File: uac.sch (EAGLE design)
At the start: 206 parts, among them Q6 2N7002CK4SST, Q7 2N7002CK4SST, U2 ADXL345, Y1 RESONATORSMD

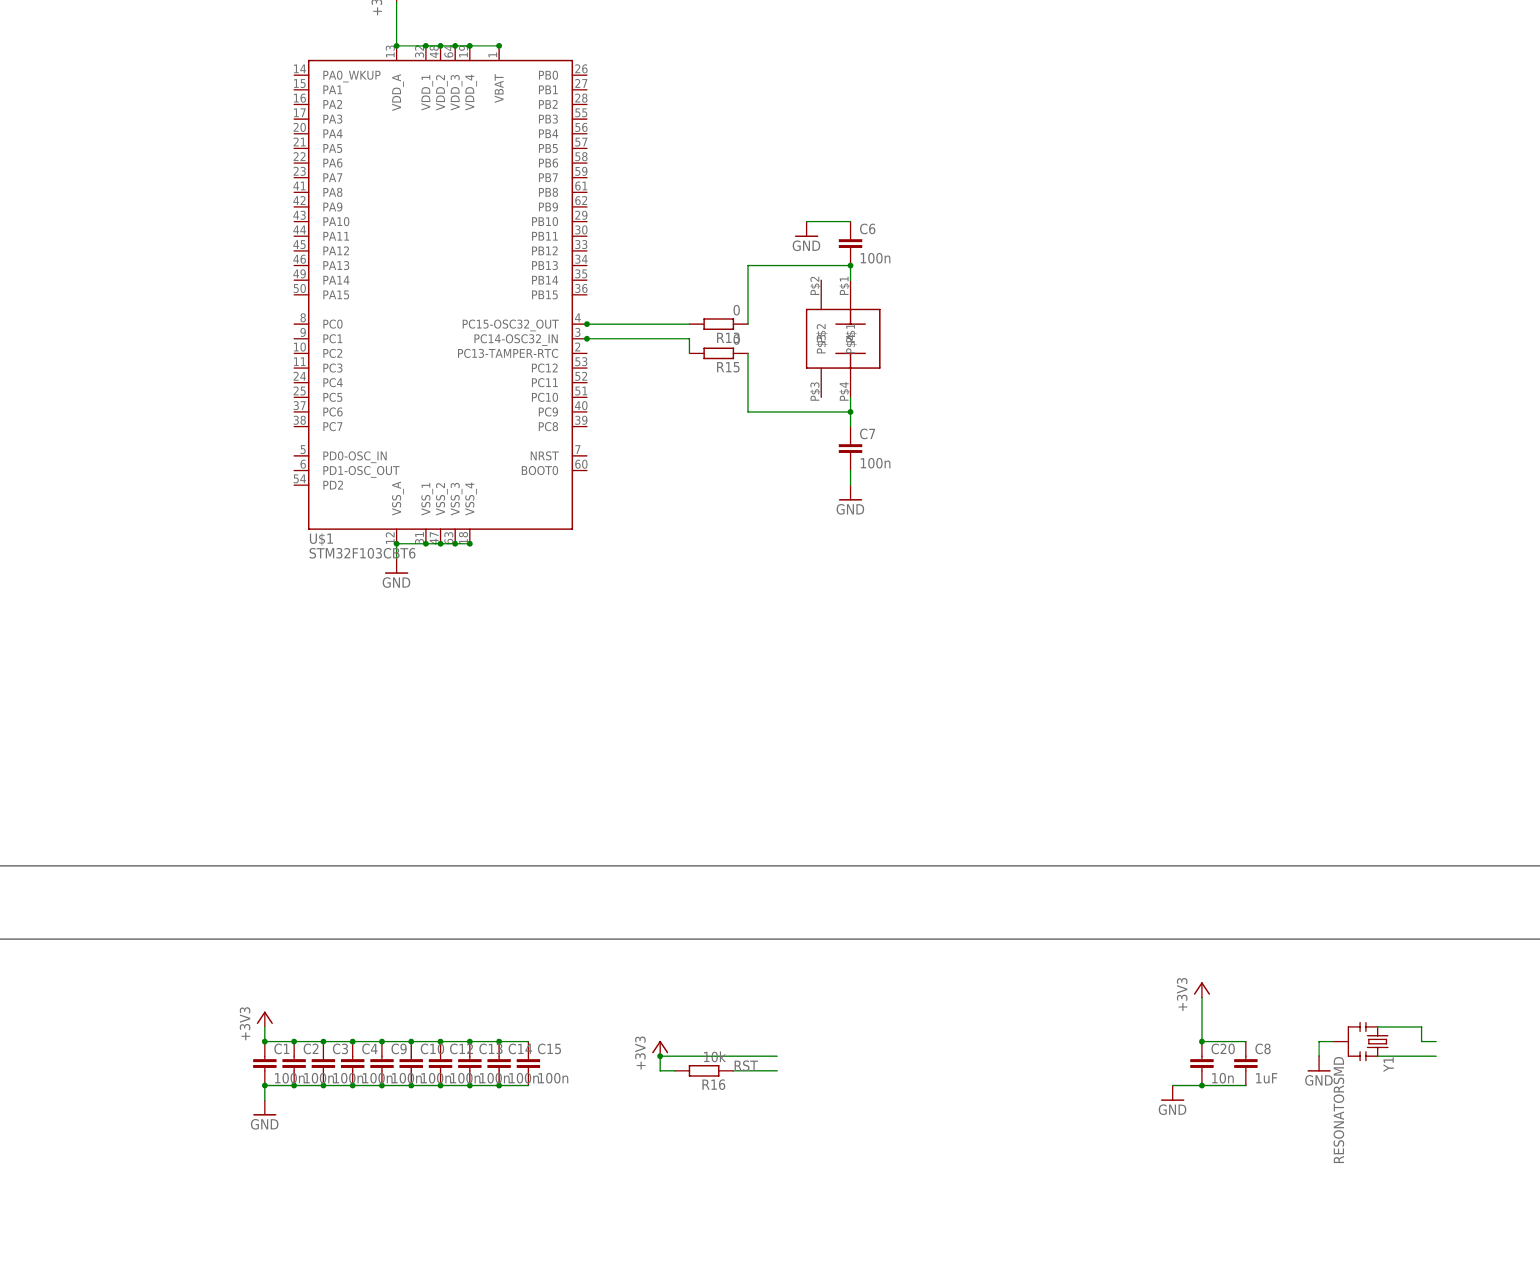
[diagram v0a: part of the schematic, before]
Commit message: connecting
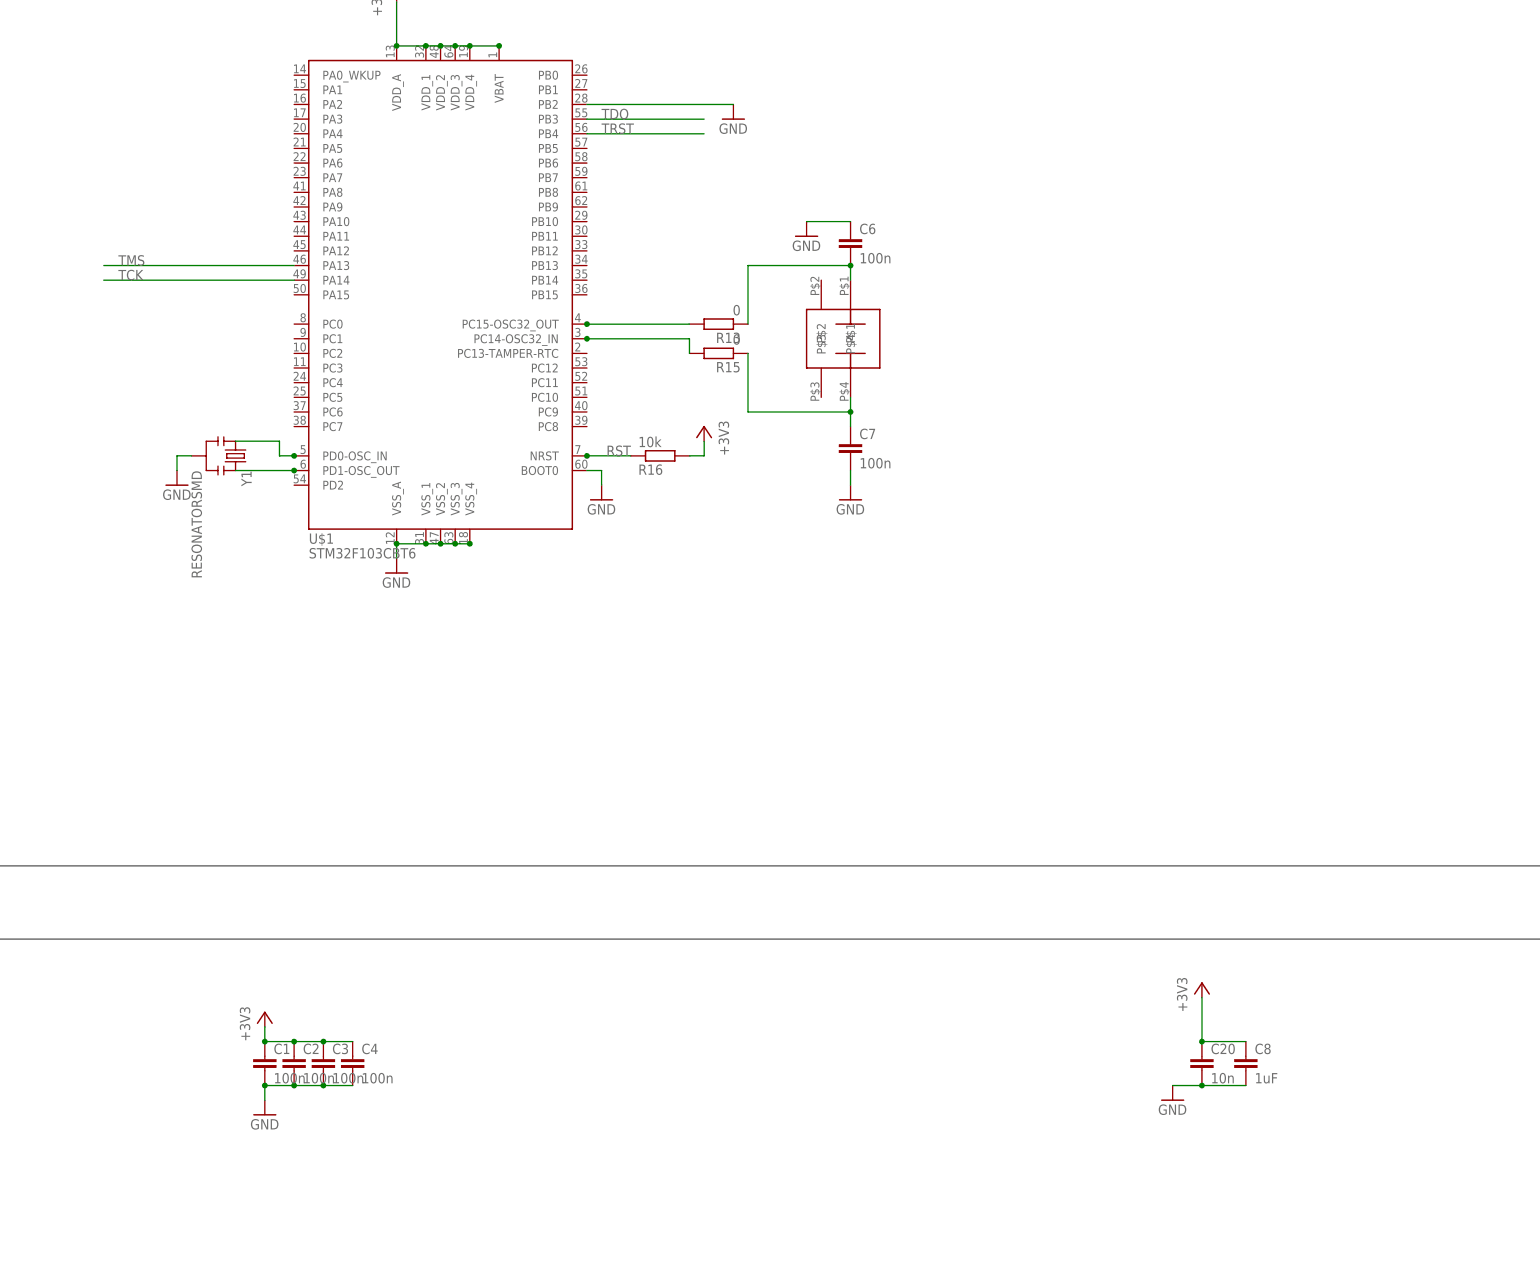
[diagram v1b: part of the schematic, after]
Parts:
- removed C10, C12, C13, C14, C15, C9: 100n, Custom components:C-EUC0603
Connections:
- net +3V3: no longer C10.1, C12.1, C13.1, C14.1, C15.1, C9.1
- net GND: now also U$1.BOOT0, U$1.PB2; no longer C10.2, C12.2, C13.2, C14.2, C15.2, C9.2
- net N$1: now also U$1.PD1-OSC_OUT
- net N$2: now also U$1.PD0-OSC_IN
- net RST: now also U$1.NRST
- net TCK: now also U$1.PA14
- net TDO: now also U$1.PB3
- net TMS: now also U$1.PA13
- net TRST: now also U$1.PB4
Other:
- moved on the sheet: R16, Y1
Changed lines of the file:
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@@
 <part name="+3V7" library="supply1" deviceset="+3V3" device=""/>
 <part name="R16" library="Custom components" deviceset="R-EU_" device="R0603" value="10k"/>
-<part name="C9" library="Custom components" deviceset="C-EU" device="C0603" value="100n"/>
-<part name="C10" library="Custom components" deviceset="C-EU" device="C0603" value="100n"/>
-<part name="C12" library="Custom components" deviceset="C-EU" device="C0603" value="100n"/>
-<part name="C13" library="Custom components" deviceset="C-EU" device="C0603" value="100n"/>
-<part name="C14" library="Custom components" deviceset="C-EU" device="C0603" value="100n"/>
-<part name="C15" library="Custom components" deviceset="C-EU" device="C0603" value="100n"/>
 <part name="GND4" library="supply1" deviceset="GND" device=""/>
 <part name="C18" library="Custom components" deviceset="C-EU" device="C0603" value="100n"/>
@@
 <part name="JP1" library="SparkFun2012" deviceset="JUMPER-2" device="SMD-NO"/>
 <part name="U$1" library="stm32" deviceset="STM32F103CBT6" device=""/>
+<part name="GND3" library="Custom components" deviceset="GND" device=""/>
+<part name="GND5" library="Custom components" deviceset="GND" device=""/>
 </parts>
 <sheets>
@@
 <instance part="C4" gate="G$1" x="147.32" y="215.9"/>
 <instance part="+3V2" gate="G$1" x="132.08" y="223.52"/>
-<instance part="Y1" gate="G$1" x="325.12" y="218.44" rot="R270"/>
-<instance part="GND2" gate="1" x="314.96" y="213.36"/>
+<instance part="Y1" gate="G$1" x="127" y="320.04" rot="R270"/>
+<instance part="GND2" gate="1" x="116.84" y="314.96"/>
 <instance part="MASTER_PROG" gate="A" x="35.56" y="203.2"/>
 <instance part="GND19" gate="1" x="12.7" y="208.28"/>
@@
 <instance part="+3V5" gate="G$1" x="154.94" y="401.32"/>
 <instance part="GND9" gate="1" x="154.94" y="299.72"/>
-<instance part="+3V7" gate="G$1" x="200.66" y="218.44"/>
-<instance part="R16" gate="G$1" x="208.28" y="213.36" rot="R180"/>
-<instance part="C9" gate="G$1" x="152.4" y="215.9"/>
-<instance part="C10" gate="G$1" x="157.48" y="215.9"/>
-<instance part="C12" gate="G$1" x="162.56" y="215.9"/>
-<instance part="C13" gate="G$1" x="167.64" y="215.9"/>
-<instance part="C14" gate="G$1" x="172.72" y="215.9"/>
-<instance part="C15" gate="G$1" x="177.8" y="215.9"/>
+<instance part="+3V7" gate="G$1" x="208.28" y="325.12" rot="MR0"/>
+<instance part="R16" gate="G$1" x="200.66" y="320.04" rot="MR180"/>
 <instance part="GND4" gate="1" x="38.1" y="20.32"/>
 <instance part="C18" gate="G$1" x="48.26" y="38.1"/>
@@
 <instance part="JP1" gate="A" x="419.1" y="134.62"/>
 <instance part="U$1" gate="G$1" x="149.86" y="363.22"/>
+<instance part="GND3" gate="1" x="190.5" y="312.42"/>
+<instance part="GND5" gate="1" x="213.36" y="378.46"/>
 </instances>
 <busses>
@@
 <pinref part="Y1" gate="G$1" pin="2"/>
 <pinref part="GND2" gate="1" pin="GND"/>
-<wire x1="317.5" y1="218.44" x2="314.96" y2="218.44" width="0.1524" layer="91"/>
-<wire x1="314.96" y1="218.44" x2="314.96" y2="215.9" width="0.1524" layer="91"/>
+<wire x1="119.38" y1="320.04" x2="116.84" y2="320.04" width="0.1524" layer="91"/>
+<wire x1="116.84" y1="320.04" x2="116.84" y2="317.5" width="0.1524" layer="91"/>
 </segment>
 <segment>
@@
 <junction x="137.16" y="210.82"/>
 <junction x="142.24" y="210.82"/>
-<junction x="147.32" y="210.82"/>
 <pinref part="GND1" gate="1" pin="GND"/>
 <wire x1="132.08" y1="208.28" x2="132.08" y2="210.82" width="0.1524" layer="91"/>
 <junction x="132.08" y="210.82"/>
-<pinref part="C15" gate="G$1" pin="2"/>
-<pinref part="C14" gate="G$1" pin="2"/>
-<wire x1="177.8" y1="210.82" x2="172.72" y2="210.82" width="0.1524" layer="91"/>
-<pinref part="C13" gate="G$1" pin="2"/>
-<wire x1="172.72" y1="210.82" x2="167.64" y2="210.82" width="0.1524" layer="91"/>
-<pinref part="C12" gate="G$1" pin="2"/>
-<wire x1="167.64" y1="210.82" x2="162.56" y2="210.82" width="0.1524" layer="91"/>
-<pinref part="C10" gate="G$1" pin="2"/>
-<wire x1="162.56" y1="210.82" x2="157.48" y2="210.82" width="0.1524" layer="91"/>
-<pinref part="C9" gate="G$1" pin="2"/>
-<wire x1="157.48" y1="210.82" x2="152.4" y2="210.82" width="0.1524" layer="91"/>
-<wire x1="152.4" y1="210.82" x2="147.32" y2="210.82" width="0.1524" layer="91"/>
-<junction x="172.72" y="210.82"/>
-<junction x="167.64" y="210.82"/>
-<junction x="162.56" y="210.82"/>
-<junction x="157.48" y="210.82"/>
-<junction x="152.4" y="210.82"/>
 </segment>
 <segment>
@@
 <junction x="167.64" y="304.8"/>
 </segment>
+<segment>
+<pinref part="U$1" gate="G$1" pin="BOOT0"/>
+<pinref part="GND3" gate="1" pin="GND"/>
+<wire x1="187.96" y1="317.5" x2="190.5" y2="317.5" width="0.1524" layer="91"/>
+<wire x1="190.5" y1="317.5" x2="190.5" y2="314.96" width="0.1524" layer="91"/>
+</segment>
+<segment>
+<pinref part="U$1" gate="G$1" pin="PB2"/>
+<pinref part="GND5" gate="1" pin="GND"/>
+<wire x1="187.96" y1="381" x2="213.36" y2="381" width="0.1524" layer="91"/>
+</segment>
 </net>
 <net name="+3V3" class="0">
@@
 <segment>
 <pinref part="+3V7" gate="G$1" pin="+3V3"/>
-<wire x1="220.98" y1="215.9" x2="200.66" y2="215.9" width="0.1524" layer="91"/>
 <pinref part="R16" gate="G$1" pin="2"/>
-<wire x1="203.2" y1="213.36" x2="200.66" y2="213.36" width="0.1524" layer="91"/>
-<wire x1="200.66" y1="213.36" x2="200.66" y2="215.9" width="0.1524" layer="91"/>
-<junction x="200.66" y="215.9"/>
+<wire x1="205.74" y1="320.04" x2="208.28" y2="320.04" width="0.1524" layer="91"/>
+<wire x1="208.28" y1="320.04" x2="208.28" y2="322.58" width="0.1524" layer="91"/>
 </segment>
 <segment>
@@
 <wire x1="132.08" y1="220.98" x2="132.08" y2="218.44" width="0.1524" layer="91"/>
 <junction x="132.08" y="218.44"/>
-<pinref part="C9" gate="G$1" pin="1"/>
-<wire x1="147.32" y1="218.44" x2="152.4" y2="218.44" width="0.1524" layer="91"/>
-<pinref part="C10" gate="G$1" pin="1"/>
-<wire x1="152.4" y1="218.44" x2="157.48" y2="218.44" width="0.1524" layer="91"/>
-<pinref part="C12" gate="G$1" pin="1"/>
-<wire x1="157.48" y1="218.44" x2="162.56" y2="218.44" width="0.1524" layer="91"/>
-<pinref part="C13" gate="G$1" pin="1"/>
-<wire x1="162.56" y1="218.44" x2="167.64" y2="218.44" width="0.1524" layer="91"/>
-<pinref part="C14" gate="G$1" pin="1"/>
-<wire x1="167.64" y1="218.44" x2="172.72" y2="218.44" width="0.1524" layer="91"/>
-<pinref part="C15" gate="G$1" pin="1"/>
-<wire x1="172.72" y1="218.44" x2="177.8" y2="218.44" width="0.1524" layer="91"/>
-<junction x="147.32" y="218.44"/>
-<junction x="152.4" y="218.44"/>
-<junction x="157.48" y="218.44"/>
-<junction x="162.56" y="218.44"/>
-<junction x="167.64" y="218.44"/>
-<junction x="172.72" y="218.44"/>
 </segment>
 <segment>
@@
 <segment>
 <pinref part="Y1" gate="G$1" pin="3"/>
-<wire x1="335.28" y1="215.9" x2="325.12" y2="215.9" width="0.1524" layer="91"/>
+<wire x1="137.16" y1="317.5" x2="127" y2="317.5" width="0.1524" layer="91"/>
+<pinref part="U$1" gate="G$1" pin="PD1-OSC_OUT"/>
+<junction x="137.16" y="317.5"/>
 </segment>
 </net>
 <net name="N$2" class="0">
 <segment>
-<wire x1="335.28" y1="218.44" x2="332.74" y2="218.44" width="0.1524" layer="91"/>
-<wire x1="332.74" y1="218.44" x2="332.74" y2="220.98" width="0.1524" layer="91"/>
+<wire x1="137.16" y1="320.04" x2="134.62" y2="320.04" width="0.1524" layer="91"/>
+<wire x1="134.62" y1="320.04" x2="134.62" y2="322.58" width="0.1524" layer="91"/>
 <pinref part="Y1" gate="G$1" pin="1"/>
-<wire x1="332.74" y1="220.98" x2="325.12" y2="220.98" width="0.1524" layer="91"/>
+<wire x1="134.62" y1="322.58" x2="127" y2="322.58" width="0.1524" layer="91"/>
+<pinref part="U$1" gate="G$1" pin="PD0-OSC_IN"/>
+<junction x="137.16" y="320.04"/>
 </segment>
 </net>
@@
 <label x="22.86" y="142.24" size="1.778" layer="95"/>
 </segment>
+<segment>
+<pinref part="U$1" gate="G$1" pin="PA13"/>
+<wire x1="137.16" y1="353.06" x2="104.14" y2="353.06" width="0.1524" layer="91"/>
+<label x="106.68" y="353.06" size="1.778" layer="95"/>
+</segment>
 </net>
 <net name="TCK" class="0">
@@
 <label x="22.86" y="139.7" size="1.778" layer="95"/>
 </segment>
+<segment>
+<pinref part="U$1" gate="G$1" pin="PA14"/>
+<wire x1="137.16" y1="350.52" x2="104.14" y2="350.52" width="0.1524" layer="91"/>
+<label x="106.68" y="350.52" size="1.778" layer="95"/>
+</segment>
 </net>
 <net name="TDO" class="0">
@@
 <label x="71.12" y="167.64" size="1.778" layer="95"/>
 </segment>
+<segment>
+<pinref part="U$1" gate="G$1" pin="PB3"/>
+<wire x1="187.96" y1="378.46" x2="208.28" y2="378.46" width="0.1524" layer="91"/>
+<label x="190.5" y="378.46" size="1.778" layer="95"/>
+</segment>
 </net>
 <net name="TRST" class="0">
@@
 <wire x1="93.98" y1="165.1" x2="68.58" y2="165.1" width="0.1524" layer="91"/>
 <label x="71.12" y="165.1" size="1.778" layer="95"/>
+</segment>
+<segment>
+<pinref part="U$1" gate="G$1" pin="PB4"/>
+<wire x1="187.96" y1="375.92" x2="208.28" y2="375.92" width="0.1524" layer="91"/>
+<label x="190.5" y="375.92" size="1.778" layer="95"/>
 </segment>
 </net>
@@
 <segment>
 <pinref part="R16" gate="G$1" pin="1"/>
-<wire x1="220.98" y1="213.36" x2="213.36" y2="213.36" width="0.1524" layer="91"/>
-<label x="213.36" y="213.36" size="1.778" layer="95"/>
-</segment>
-</net>
+<wire x1="187.96" y1="320.04" x2="195.58" y2="320.04" width="0.1524" layer="91"/>
+<label x="195.58" y="320.04" size="1.778" layer="95" rot="MR0"/>
+<pinref part="U$1" gate="G$1" pin="NRST"/>
+<junction x="187.96" y="320.04"/>
+</segment>
+</net>
